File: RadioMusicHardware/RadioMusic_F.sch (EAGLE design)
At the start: 30 parts, among them X1 VERT_SD_CARD_REV2

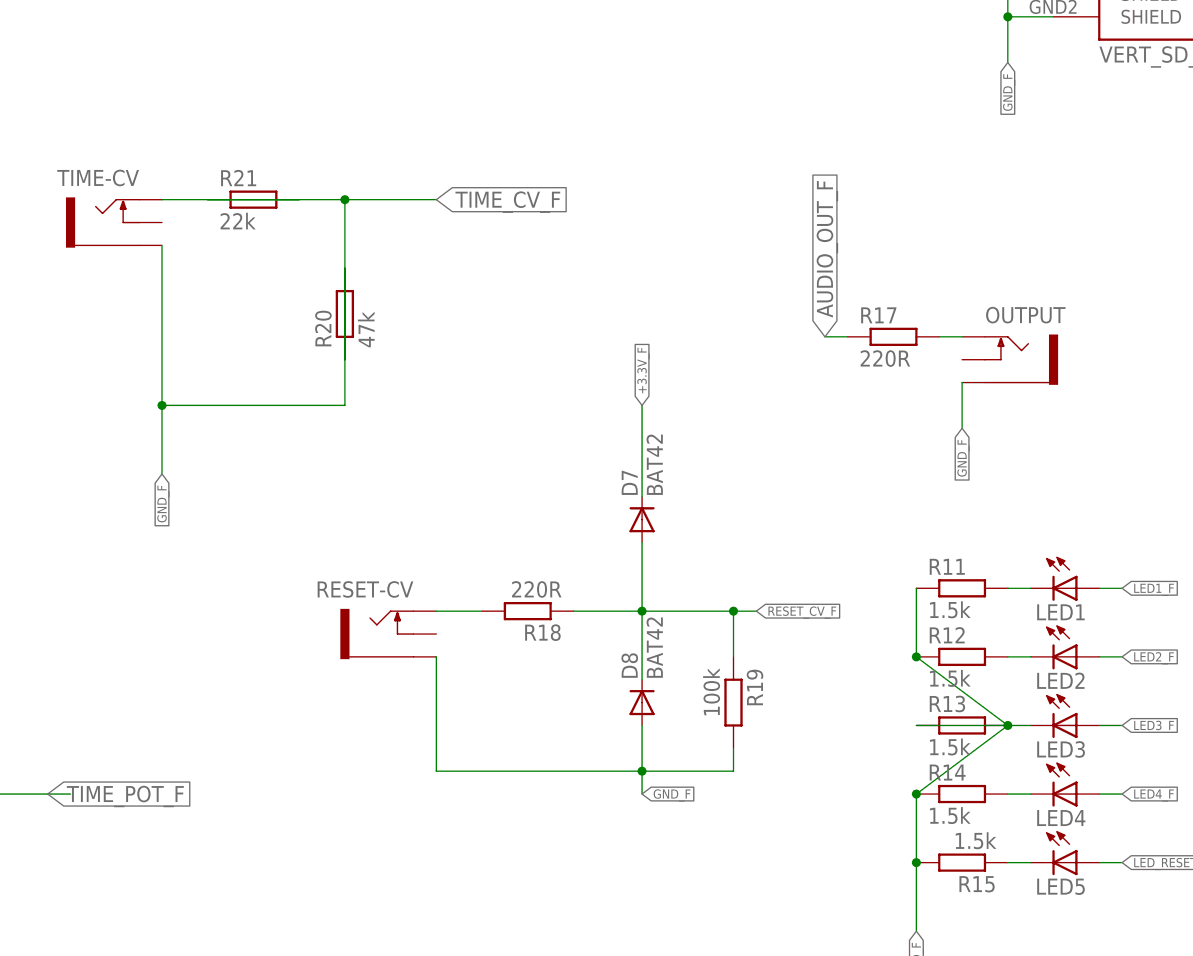
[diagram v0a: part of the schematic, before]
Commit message: 3.1 Hardware Finalised
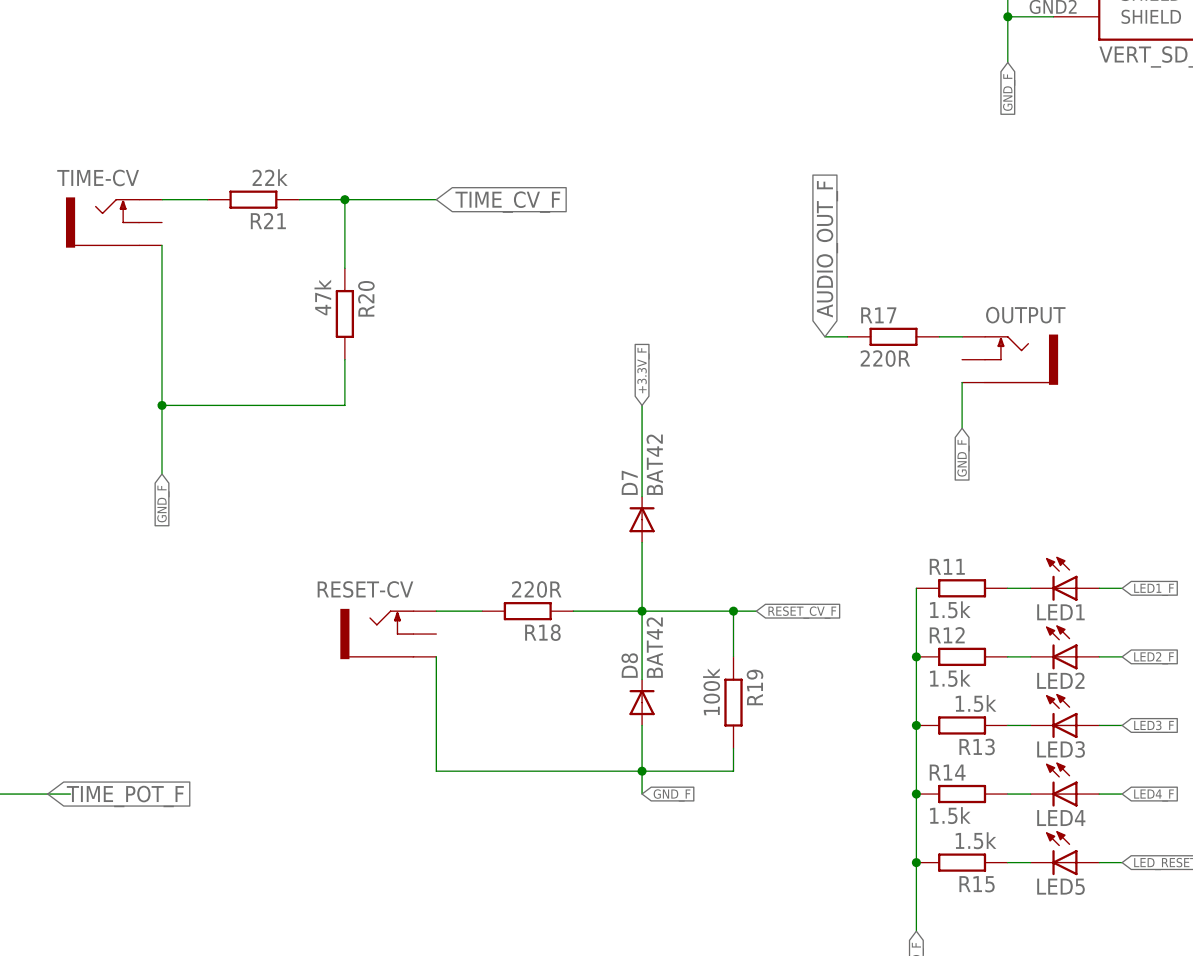
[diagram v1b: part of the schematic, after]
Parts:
- R11, R12, R14, R15, R17, R18, R19, R8, R9: device TomW:R-EU_STANDARD_RESISTOR -> MusicThingModular:RESISTOR7MM
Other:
- moved on the sheet: R13, R20, R21
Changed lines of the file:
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@@
 <?xml version="1.0" encoding="utf-8"?>
 <!DOCTYPE eagle SYSTEM "eagle.dtd">
-<eagle version="7.4.0">
+<eagle version="7.2.0">
 <drawing>
 <settings>
@@
 <part name="RESET-CV" library="MusicThingModular" deviceset="THONKICONN" device="NEW" value="THONKICONNNEW"/>
 <part name="OUTPUT" library="MusicThingModular" deviceset="THONKICONN" device="NEW" value="THONKICONNNEW"/>
-<part name="R9" library="TomW" deviceset="R-EU_" device="STANDARD_RESISTOR" value="47k"/>
+<part name="R9" library="MusicThingModular" deviceset="RESISTOR" device="7MM" value="47k"/>
 <part name="R10" library="MusicThingModular" deviceset="RESISTOR" device="VERTICAL" value="22k"/>
-<part name="R17" library="TomW" deviceset="R-EU_" device="STANDARD_RESISTOR" value="220R"/>
+<part name="R17" library="MusicThingModular" deviceset="RESISTOR" device="7MM" value="220R"/>
 <part name="TIME-POT" library="TomW" deviceset="ALPHA-9MM" device="A" technology="F2" value="50k"/>
 <part name="TIME-CV" library="MusicThingModular" deviceset="THONKICONN" device="NEW" value="THONKICONNNEW"/>
@@
 <part name="D7" library="diode" deviceset="BAT81" device="" value="BAT42"/>
 <part name="D8" library="diode" deviceset="BAT81" device="" value="BAT42"/>
-<part name="R19" library="TomW" deviceset="R-EU_" device="STANDARD_RESISTOR" value="100k"/>
-<part name="R18" library="TomW" deviceset="R-EU_" device="STANDARD_RESISTOR" value="220R"/>
+<part name="R19" library="MusicThingModular" deviceset="RESISTOR" device="7MM" value="100k"/>
+<part name="R18" library="MusicThingModular" deviceset="RESISTOR" device="7MM" value="220R"/>
 <part name="RESET" library="TomW" deviceset="D6_PUSH_SWITCH" device="" value="D6_PUSH_SWITCH"/>
-<part name="R8" library="TomW" deviceset="R-EU_" device="STANDARD_RESISTOR" value="10k"/>
+<part name="R8" library="MusicThingModular" deviceset="RESISTOR" device="7MM" value="10k"/>
 <part name="LED1" library="TomW" deviceset="LED" device="3MM"/>
 <part name="LED2" library="TomW" deviceset="LED" device="3MM"/>
 <part name="LED3" library="TomW" deviceset="LED" device="3MM"/>
 <part name="LED4" library="TomW" deviceset="LED" device="3MM"/>
-<part name="R11" library="TomW" deviceset="R-EU_" device="STANDARD_RESISTOR" value="1.5k"/>
-<part name="R12" library="TomW" deviceset="R-EU_" device="STANDARD_RESISTOR" value="1.5k"/>
+<part name="R11" library="MusicThingModular" deviceset="RESISTOR" device="7MM" value="1.5k"/>
+<part name="R12" library="MusicThingModular" deviceset="RESISTOR" device="7MM" value="1.5k"/>
 <part name="R13" library="MusicThingModular" deviceset="RESISTOR" device="VERTICAL" value="1.5k"/>
-<part name="R14" library="TomW" deviceset="R-EU_" device="STANDARD_RESISTOR" value="1.5k"/>
+<part name="R14" library="MusicThingModular" deviceset="RESISTOR" device="7MM" value="1.5k"/>
 <part name="X1" library="TomW" deviceset="VERT_SD_CARD_REV2" device=""/>
 <part name="LED5" library="TomW" deviceset="LED" device="3MM"/>
-<part name="R15" library="TomW" deviceset="R-EU_" device="STANDARD_RESISTOR" value="1.5k"/>
+<part name="R15" library="MusicThingModular" deviceset="RESISTOR" device="7MM" value="1.5k"/>
 <part name="JP2" library="SparkFun-Connectors" deviceset="M11" device="PTH" value="M11PTH"/>
 <part name="JP4" library="SparkFun-Connectors" deviceset="M07" device=""/>
@@
 <instance part="TIME-POT" gate="G$1" x="30.48" y="22.86"/>
 <instance part="TIME-CV" gate="G$1" x="50.8" y="86.36" rot="MR0"/>
-<instance part="R20" gate="G$1" x="76.2" y="76.2" rot="R90"/>
-<instance part="R21" gate="G$1" x="66.04" y="88.9"/>
+<instance part="R20" gate="G$1" x="76.2" y="76.2" rot="R270"/>
+<instance part="R21" gate="G$1" x="66.04" y="88.9" rot="R180"/>
 <instance part="D7" gate="1" x="109.22" y="53.34" rot="R90"/>
 <instance part="D8" gate="1" x="109.22" y="33.02" rot="R90"/>
@@
 <instance part="R11" gate="G$1" x="144.78" y="45.72"/>
 <instance part="R12" gate="G$1" x="144.78" y="38.1"/>
-<instance part="R13" gate="G$1" x="144.78" y="30.48"/>
+<instance part="R13" gate="G$1" x="144.78" y="30.48" rot="R180"/>
 <instance part="R14" gate="G$1" x="144.78" y="22.86"/>
 <instance part="X1" gate="G$1" x="162.56" y="121.92"/>
@@
 <pinref part="LED3" gate="G$1" pin="C"/>
 <pinref part="R13" gate="G$1" pin="1"/>
-<wire x1="139.7" y1="30.48" x2="152.4" y2="30.48" width="0.1524" layer="91"/>
+<wire x1="149.86" y1="30.48" x2="152.4" y2="30.48" width="0.1524" layer="91"/>
 </segment>
 </net>
@@
 <pinref part="R20" gate="G$1" pin="2"/>
 <wire x1="55.88" y1="66.04" x2="55.88" y2="83.82" width="0.1524" layer="91"/>
-<wire x1="76.2" y1="81.28" x2="76.2" y2="66.04" width="0.1524" layer="91"/>
+<wire x1="76.2" y1="71.12" x2="76.2" y2="66.04" width="0.1524" layer="91"/>
 <wire x1="76.2" y1="66.04" x2="55.88" y2="66.04" width="0.1524" layer="91"/>
 <junction x="55.88" y="66.04"/>
@@
 <pinref part="R11" gate="G$1" pin="1"/>
 <pinref part="R12" gate="G$1" pin="1"/>
-<wire x1="139.7" y1="38.1" x2="149.86" y2="30.48" width="0.1524" layer="91"/>
+<wire x1="139.7" y1="38.1" x2="139.7" y2="30.48" width="0.1524" layer="91"/>
 <junction x="139.7" y="38.1"/>
 <pinref part="R13" gate="G$1" pin="2"/>
-<wire x1="149.86" y1="30.48" x2="139.7" y2="22.86" width="0.1524" layer="91"/>
-<junction x="149.86" y="30.48"/>
+<wire x1="139.7" y1="30.48" x2="139.7" y2="22.86" width="0.1524" layer="91"/>
+<junction x="139.7" y="30.48"/>
 <pinref part="R14" gate="G$1" pin="1"/>
 <wire x1="139.7" y1="22.86" x2="139.7" y2="15.24" width="0.1524" layer="91"/>
@@
 <segment>
 <pinref part="R21" gate="G$1" pin="1"/>
-<wire x1="60.96" y1="88.9" x2="76.2" y2="88.9" width="0.1524" layer="91"/>
+<wire x1="71.12" y1="88.9" x2="76.2" y2="88.9" width="0.1524" layer="91"/>
 <pinref part="R20" gate="G$1" pin="1"/>
 <wire x1="76.2" y1="88.9" x2="86.36" y2="88.9" width="0.1524" layer="91"/>
-<wire x1="76.2" y1="71.12" x2="76.2" y2="88.9" width="0.1524" layer="91"/>
+<wire x1="76.2" y1="81.28" x2="76.2" y2="88.9" width="0.1524" layer="91"/>
 <junction x="76.2" y="88.9"/>
 <label x="86.36" y="88.9" size="1.778" layer="95" xref="yes"/>
@@
 <pinref part="TIME-CV" gate="G$1" pin="TIP"/>
 <pinref part="R21" gate="G$1" pin="2"/>
-<wire x1="71.12" y1="88.9" x2="55.88" y2="88.9" width="0.1524" layer="91"/>
-</segment>
-</net>
+<wire x1="60.96" y1="88.9" x2="55.88" y2="88.9" width="0.1524" layer="91"/>
+</segment>
+</net>
